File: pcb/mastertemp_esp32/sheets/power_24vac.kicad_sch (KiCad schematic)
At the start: 12 parts, among them J1 POWER_24VAC_3P, U1 LM5164_100V_BUCK_5V, U2 3V3_BUCK_OR_REGULATOR_TBD, U3 3V3_RESET_SUPERVISOR_TBD

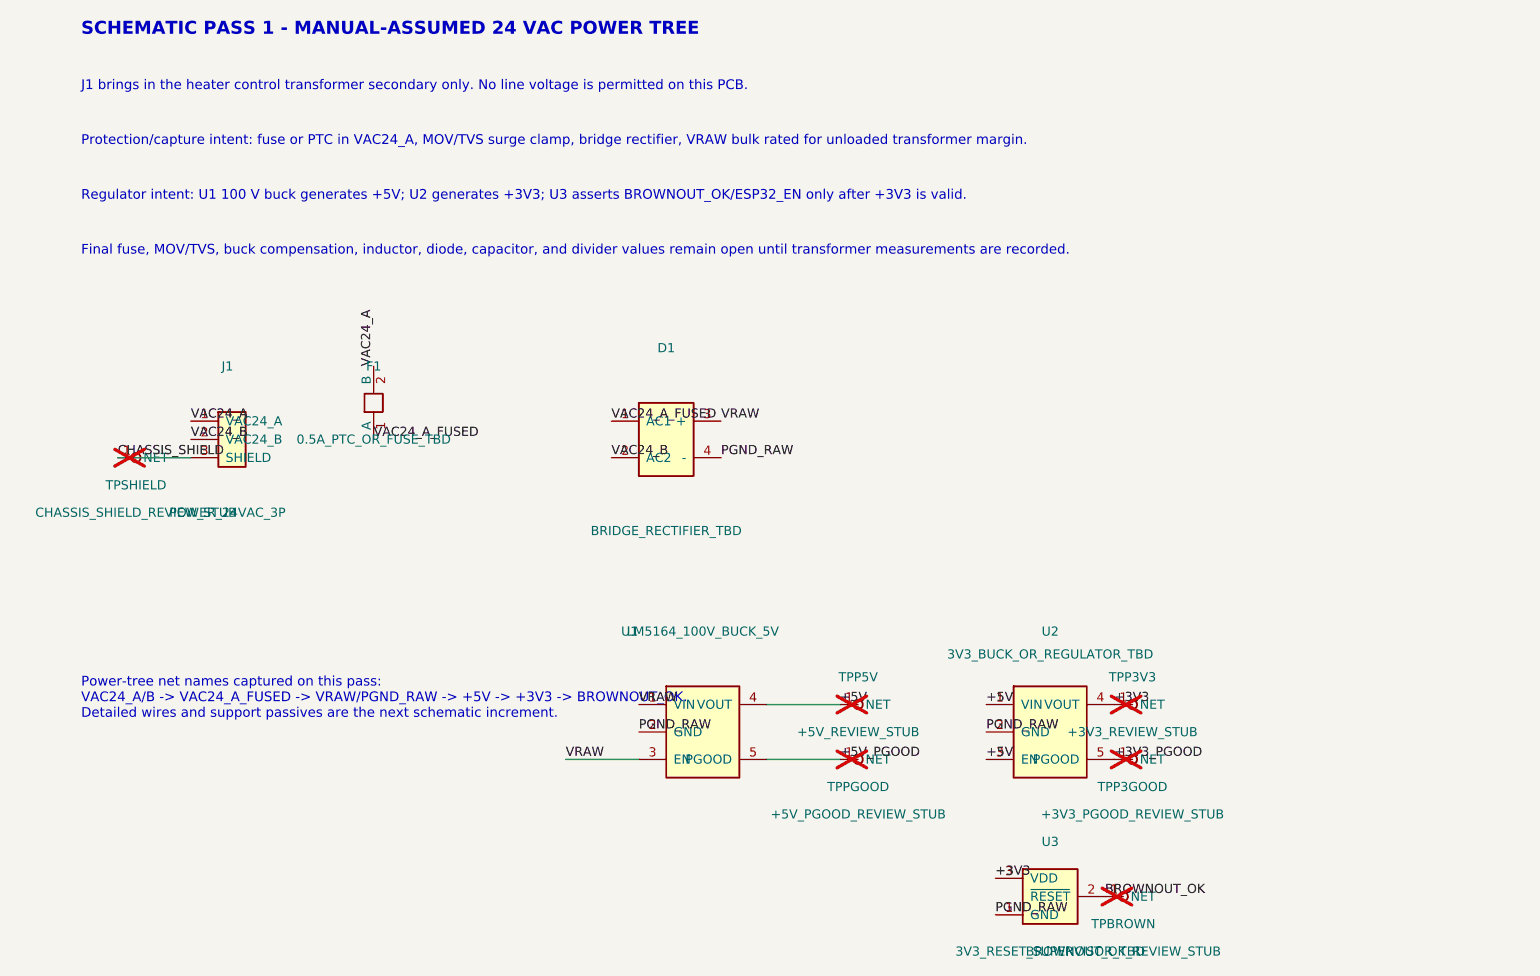
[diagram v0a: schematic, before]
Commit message: AI
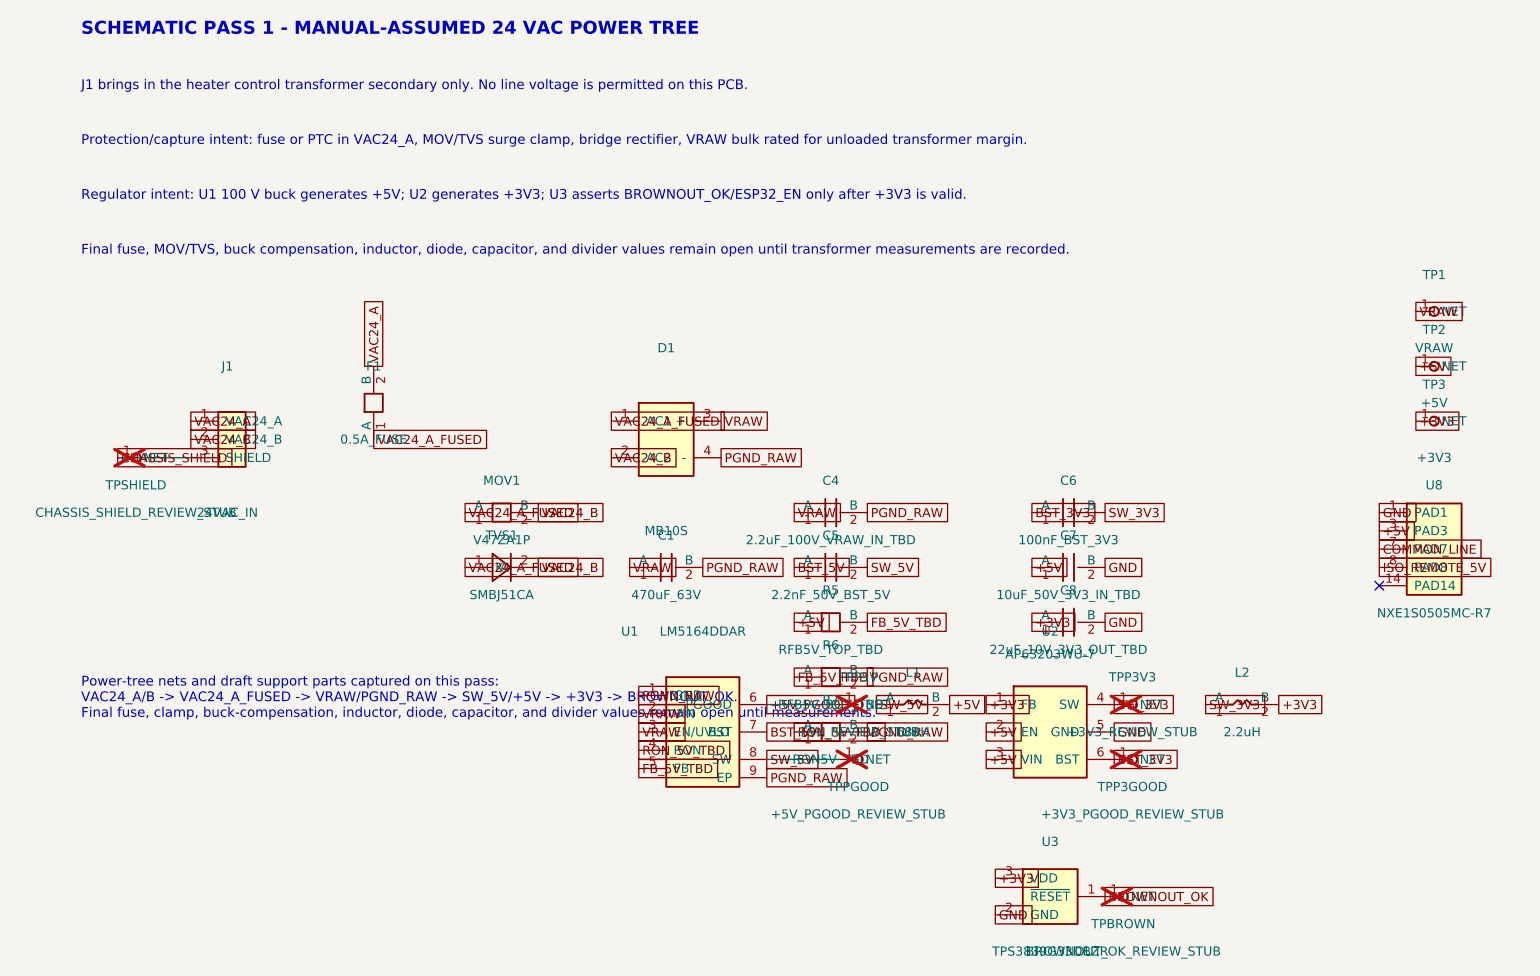
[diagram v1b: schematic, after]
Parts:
- added C1: 470uF_63V, Capacitor_THT:CP_Radial_D10.0mm_P5.00mm, symbol mastertemp_esp32:Capacitor_2pin
- added C4: 2.2uF_100V_VRAW_IN_TBD, Capacitor_SMD:C_1210_3225Metric, symbol mastertemp_esp32:Capacitor_2pin
- added C5: 2.2nF_50V_BST_5V, Capacitor_SMD:C_0603_1608Metric, symbol mastertemp_esp32:Capacitor_2pin
- added C6: 100nF_BST_3V3, Capacitor_SMD:C_0603_1608Metric, symbol mastertemp_esp32:Capacitor_2pin
- added C7: 10uF_50V_3V3_IN_TBD, Capacitor_SMD:C_1210_3225Metric, symbol mastertemp_esp32:Capacitor_2pin
- added C8: 22uF_10V_3V3_OUT_TBD, Capacitor_SMD:C_0805_2012Metric, symbol mastertemp_esp32:Capacitor_2pin
- added L1: 68uH, Inductor_SMD:L_12x12mm_H8mm, symbol mastertemp_esp32:Inductor_2pin
- added L2: 2.2uH, Inductor_SMD:L_Vishay_IFSC-1515AH_4x4x1.8mm, symbol mastertemp_esp32:Inductor_2pin
- added MOV1: V47ZA1P, Varistor:RV_Disc_D7mm_W3.9mm_P5mm, symbol mastertemp_esp32:Resistor_2pin
- added R5: RFB5V_TOP_TBD, Resistor_SMD:R_0805_2012Metric, symbol mastertemp_esp32:Resistor_2pin
- added R6: RFB5V_BOT_TBD, Resistor_SMD:R_0805_2012Metric, symbol mastertemp_esp32:Resistor_2pin
- added R7: RON5V_TBD, Resistor_SMD:R_0805_2012Metric, symbol mastertemp_esp32:Resistor_2pin
- added TP1: VRAW, TestPoint_Pad_D2.0mm, symbol mastertemp_esp32:NetStub_1pin
- added TP2: +5V, TestPoint_Pad_D2.0mm, symbol mastertemp_esp32:NetStub_1pin
- added TP3: +3V3, TestPoint_Pad_D2.0mm, symbol mastertemp_esp32:NetStub_1pin
- added TVS1: SMBJ51CA, Diode_SMD:D_SMB, symbol mastertemp_esp32:Diode_2pin
- added U8: NXE1S0505MC-R7, Converter_DCDC:Converter_DCDC_Murata_NXExSxxxxMC_SMD, symbol mastertemp_esp32:Uncommitted_NXE5
- D1: value BRIDGE_RECTIFIER_TBD -> MB10S; footprint (none) -> Diode_SMD:Diode_Bridge_Vishay_MBLS
- F1: value 0.5A_PTC_OR_FUSE_TBD -> 0.5A_FUSE; footprint (none) -> Fuse:Fuse_1206_3216Metric
- J1: value POWER_24VAC_3P -> 24VAC_IN; footprint Connector_Phoenix_MC_HighVoltage:PhoenixContact_MSTBA_2,5_3-G-5,08_1x03_P5.08mm_Horizontal -> Connector_Phoenix_MSTB:PhoenixContact_MSTBA_2,5_3-G-5,08_1x03_P5.08mm_Horizontal
- U1: value LM5164_100V_BUCK_5V -> LM5164DDAR; footprint Package_DFN_QFN:Texas_S-PVSON-N10 -> Package_SO:TI_SO-PowerPAD-8; symbol mastertemp_esp32:PowerBuck_5pin -> mastertemp_esp32:LM5164_DDA8
- U2: value 3V3_BUCK_OR_REGULATOR_TBD -> AP63203WU-7; symbol mastertemp_esp32:PowerBuck_5pin -> mastertemp_esp32:AP63203_TSOT26
- U3: value 3V3_RESET_SUPERVISOR_TBD -> TPS3839G33DBZR; footprint Package_TO_SOT_SMD:SOT-23 -> Package_TO_SOT_SMD:SOT-23-3
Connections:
- net +3V3: now also U2.1 (FB), C8.1 (A), L2.2 (B), TP3.1 (NET); no longer TPP3V3.1 (NET), U2.4 (VOUT)
- net +5V: now also U2.2 (EN), C7.1 (A), L1.2 (B), R5.1 (A), TP2.1 (NET), U8.3 (PAD3); no longer TPP5V.1 (NET), U1.4 (VOUT), U2.1 (VIN)
- net +5V_PGOOD: now also TPP5V.1 (NET), U1.6 (PGOOD); no longer TPPGOOD.1 (NET), U1.5 (PGOOD)
- net BROWNOUT_OK: now also U3.1 (~{RESET}); no longer U3.2 (~{RESET})
- net PGND_RAW: now also U1.1 (GND), U1.9 (EP), C1.2 (B), C4.2 (B), R6.2 (B), R7.2 (B); no longer U1.2 (GND), U2.2 (GND), U3.1 (GND)
- net VAC24_A_FUSED: now also MOV1.1 (A), TVS1.1 (A)
- net VAC24_B: now also MOV1.2 (B), TVS1.2 (K)
- net VRAW: now also U1.2 (VIN), C1.1 (A), C4.1 (A), TP1.1 (NET); no longer U1.1 (VIN)
- net +3V3_PGOOD renamed BST_3V3
- net BST_3V3: now also U2.6 (BST), C6.1 (A); no longer U2.5 (PGOOD)
- new net BST_5V: C5.1 (A), U1.7 (BST)
- new net COMMON_LINE: U8.7 (PAD7)
- new net FB_5V_TBD: R5.2 (B), R6.1 (A), U1.5 (FB)
- new net GND: C7.2 (B), C8.2 (B), U2.5 (GND), U3.2 (GND), U8.1 (PAD1)
- new net ISO_REMOTE_5V: U8.8 (PAD8)
- new net RON_5V_TBD: R7.1 (A), U1.4 (RON)
- new net SW_3V3: C6.2 (B), L2.1 (A), TPP3V3.1 (NET), U2.4 (SW)
- new net SW_5V: C5.2 (B), L1.1 (A), TPPGOOD.1 (NET), U1.8 (SW)
- no-connect marks 0 -> 1
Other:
- note added: "Power-tree nets and draft support parts captured on this pass: VAC24_A/B -> VAC24_A_FUSED -> VRAW/PGND_RAW -> SW_5V/+5V -> +3V3 -> BROWNOUT_OK. Final fuse, clamp, buck-compensation, inductor, diode, capacitor, and divider values remain open until measurements."
- note removed: "Power-tree net names captured on this pass: VAC24_A/B -> VAC24_A_FUSED -> VRAW/PGND_RAW -> +5V -> +3V3 -> BROWNOUT_OK. Detailed wires and support passives are the next schematic increment."
